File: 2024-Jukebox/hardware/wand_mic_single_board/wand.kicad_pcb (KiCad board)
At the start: 4 copper layers, 17.5 x 47 mm, 52 parts, among them J1 USB_C_Receptacle_USB2.0, J10 Conn_01x03, J4 Conn_01x02, J6 Conn_01x01, J9 Conn_01x02, Q1 MUN5214DW1T1G, Q3 CJ3139K, U1 CP2104, U2 ESP32-PICO-D4, U3 ICM-20948, U4 TP4065-4.2V, U5 TLV76718DRVx, U6 LY68L6400SLIT, U7 PCA9306, U9 TLV76733DRVx

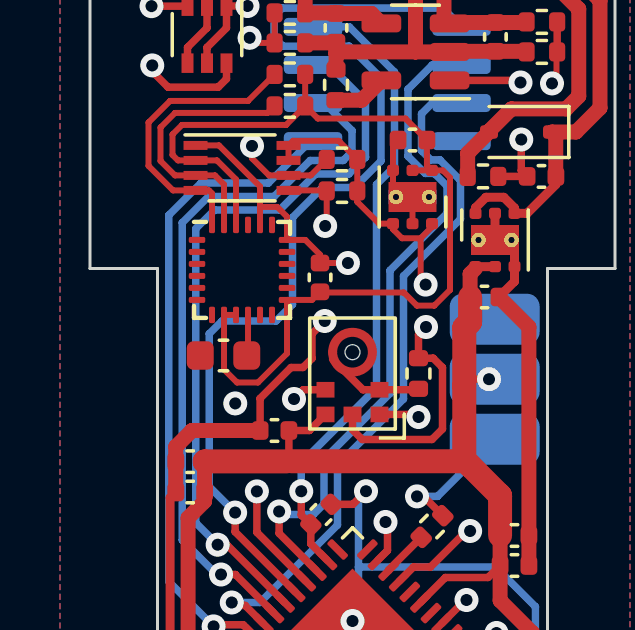
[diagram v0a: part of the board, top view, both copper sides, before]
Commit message: Update wand.kicad_pcb
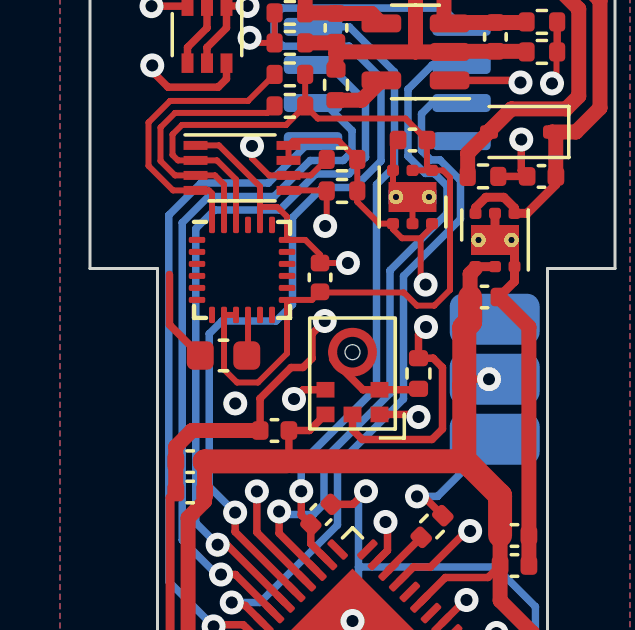
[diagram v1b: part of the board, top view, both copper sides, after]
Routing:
- net GND: track 147.2 -> 150.3 mm
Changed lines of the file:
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@@
   (segment (start 10.85 14.35) (end 10.85 13.2) (width 0.5) (layer "F.Cu") (net 5))
   (segment (start 5.667157 22.547157) (end 5.667157 21.947157) (width 0.2) (layer "F.Cu") (net 5))
+  (segment (start 3.675 26.9) (end 2.65 25.875) (width 0.25) (layer "F.Cu") (net 5))
   (segment (start 12.49 6.01) (end 13.07 5.43) (width 0.25) (layer "F.Cu") (net 5))
   (segment (start 7.177156 23.047157) (end 7.667157 23.537158) (width 0.2) (layer "F.Cu") (net 5))
@@
   (segment (start 9.1 28.042) (end 8.0875 27.0295) (width 0.25) (layer "F.Cu") (net 5))
   (segment (start 5.55 6.01) (end 5.01 6.01) (width 0.25) (layer "F.Cu") (net 5))
+  (segment (start 2.65 25.875) (end 2.65 24.2) (width 0.25) (layer "F.Cu") (net 5))
   (segment (start 6.238517 21.947157) (end 5.667157 21.947157) (width 0.2) (layer "F.Cu") (net 5))
   (segment (start 2.24 11.97) (end 3.67 10.54) (width 0.25) (layer "F.Cu") (net 5))

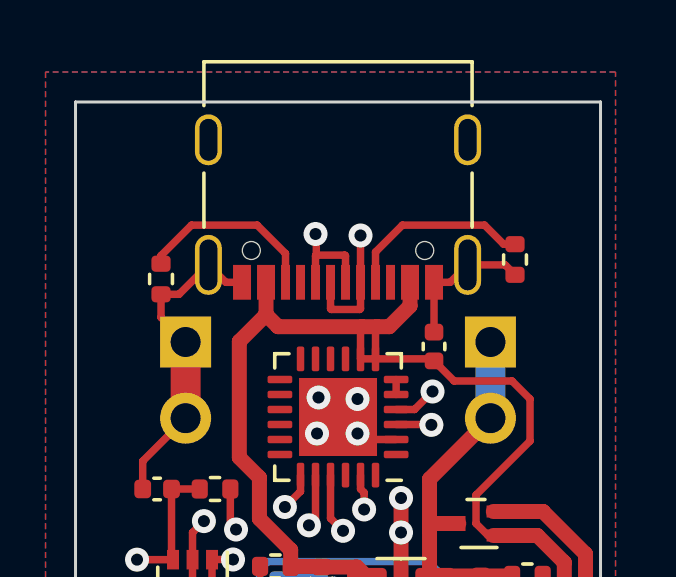
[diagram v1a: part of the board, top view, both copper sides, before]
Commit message: Updated gerbers
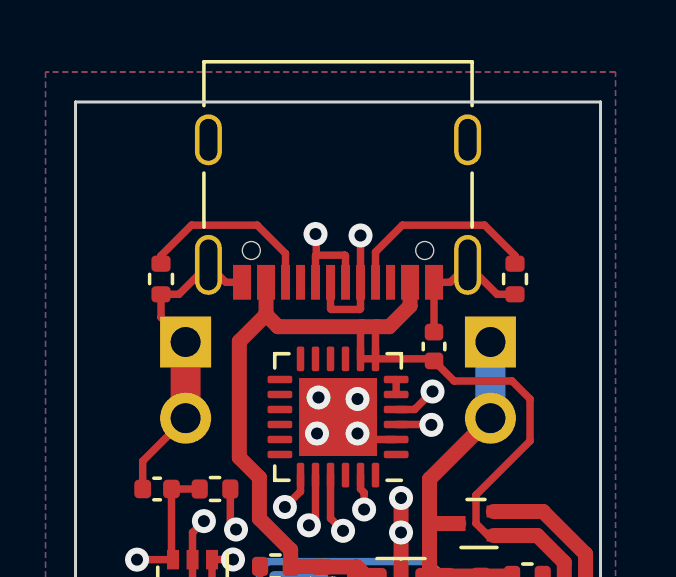
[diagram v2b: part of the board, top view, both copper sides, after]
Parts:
- moved R2 0.65 mm to (14.7, 5.90)
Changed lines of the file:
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@@
   )
   (footprint "Resistor_SMD:R_0402_1005Metric" (layer "F.Cu")
-    (at 14.65 5.25 -90)
+    (at 14.65 5.9 -90)
     (descr "Resistor SMD 0402 (1005 Metric), square (rectangular) end terminal, IPC_7351 nominal, (Body size source: IPC-SM-782 page 72, https://www.pcb-3d.com/wordpress/wp-content/uploads/ipc-sm-782a_amendment_1_and_2.pdf), generated with kicad-footprint-generator")
     (tags "resistor")
@@
   (segment (start 10.1 20.73) (end 10.1 19.8875) (width 0.2) (layer "F.Cu") (net 5))
   (segment (start 10.85 16.78) (end 10.85 14.35) (width 0.5) (layer "F.Cu") (net 5))
+  (segment (start 14.05 6.41) (end 13.07 5.43) (width 0.25) (layer "F.Cu") (net 5))
   (segment (start 9.65 28.042) (end 9.1 28.042) (width 0.25) (layer "F.Cu") (net 5))
   (segment (start 10.6875 11.25) (end 9.5 11.25) (width 0.25) (layer "F.Cu") (net 5))
@@
   (segment (start 12.0075 16.76) (end 11.9875 16.78) (width 0.5) (layer "F.Cu") (net 5))
   (segment (start 14.4 41.525) (end 14.4 42.5) (width 0.5) (layer "F.Cu") (net 5))
-  (segment (start 13.07 5.43) (end 14.32 5.43) (width 0.25) (layer "F.Cu") (net 5))
   (segment (start 14.63 25.95) (end 13.63 24.95) (width 0.5) (layer "F.Cu") (net 5))
   (segment (start 3.45 6.41) (end 4.43 5.43) (width 0.25) (layer "F.Cu") (net 5))
@@
   (segment (start 9.2 31.4245) (end 8.763911 31.860589) (width 0.25) (layer "F.Cu") (net 5))
   (segment (start 13.5 22.1625) (end 13.5 23.05) (width 0.3) (layer "F.Cu") (net 5))
+  (segment (start 14.65 6.41) (end 14.05 6.41) (width 0.25) (layer "F.Cu") (net 5))
   (segment (start 11.95 6.01) (end 12.49 6.01) (width 0.25) (layer "F.Cu") (net 5))
-  (segment (start 14.32 5.43) (end 14.65 5.76) (width 0.25) (layer "F.Cu") (net 5))
   (segment (start 14.4 42.5) (end 12.928822 42.5) (width 0.5) (layer "F.Cu") (net 5))
   (segment (start 11.95 7.67) (end 11.95 6.01) (width 0.25) (layer "F.Cu") (net 5))
@@
   (segment (start 9.55 27.977208) (end 9.55 21.2) (width 0.25) (layer "B.Cu") (net 17))
   (segment (start 10.15 17.45) (end 8.645 15.945) (width 0.25) (layer "B.Cu") (net 17))
-  (segment (start 13.634999 4.105) (end 14.269999 4.74) (width 0.25) (layer "F.Cu") (net 18))
-  (segment (start 13.634999 4.105) (end 10.895 4.105) (width 0.25) (layer "F.Cu") (net 18))
-  (segment (start 10.895 4.105) (end 10 5) (width 0.25) (layer "F.Cu") (net 18))
-  (segment (start 14.269999 4.74) (end 14.65 4.74) (width 0.25) (layer "F.Cu") (net 18))
-  (segment (start 10 5) (end 10 6.01) (width 0.25) (layer "F.Cu") (net 18))
+  (segment (start 10 5) (end 10.895 4.105) (width 0.25) (layer "F.Cu") (net 18))
+  (segment (start 13.634999 4.105) (end 14.65 5.120001) (width 0.25) (layer "F.Cu") (net 18))
+  (segment (start 10.895 4.105) (end 13.634999 4.105) (width 0.25) (layer "F.Cu") (net 18))
+  (segment (start 14.65 5.120001) (end 14.65 5.39) (width 0.25) (layer "F.Cu") (net 18))
+  (segment (start 10 6.01) (end 10 5) (width 0.25) (layer "F.Cu") (net 18))
   (segment (start 8.025 4.425) (end 8 4.4) (width 0.25) (layer "F.Cu") (net 19))
   (segment (start 8 6.01) (end 8 5.13) (width 0.25) (layer "F.Cu") (net 19))
